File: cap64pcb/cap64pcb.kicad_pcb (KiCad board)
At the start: 2 copper layers, 91.6 x 12 mm, 29 parts, among them J1 SM05B_SURS_TF, Q1 BSS138, Q2 BSS138, U1 MPR121QR2, U2 SPX3819M5-L-3.3

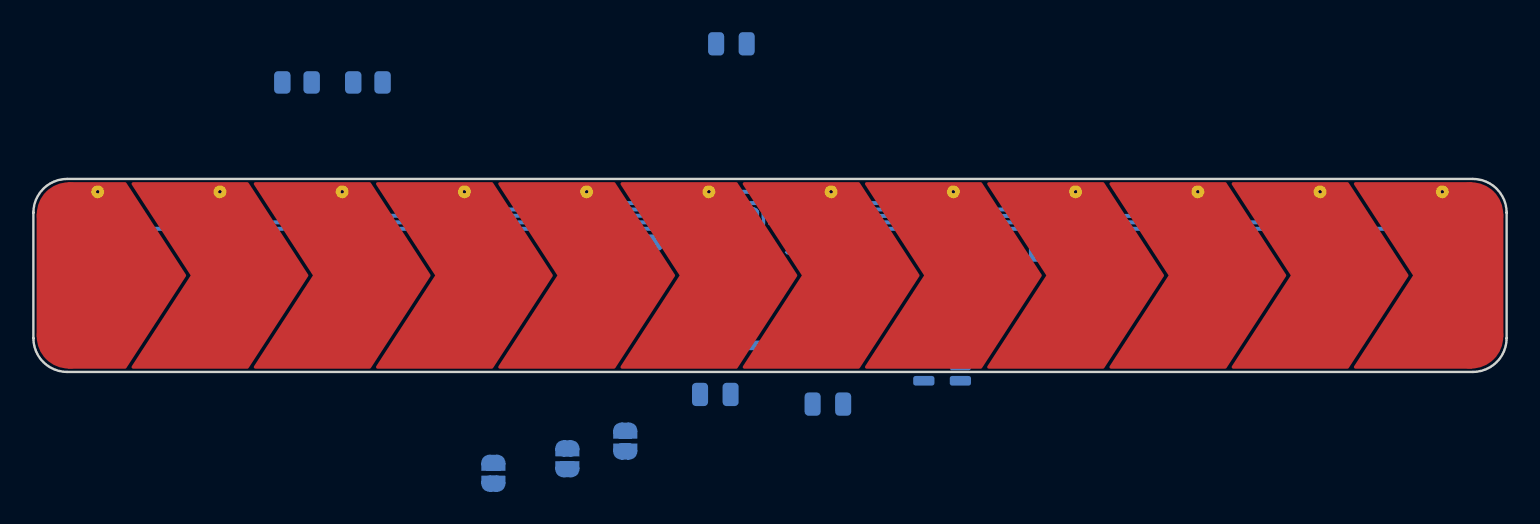
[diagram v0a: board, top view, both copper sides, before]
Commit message: test traces
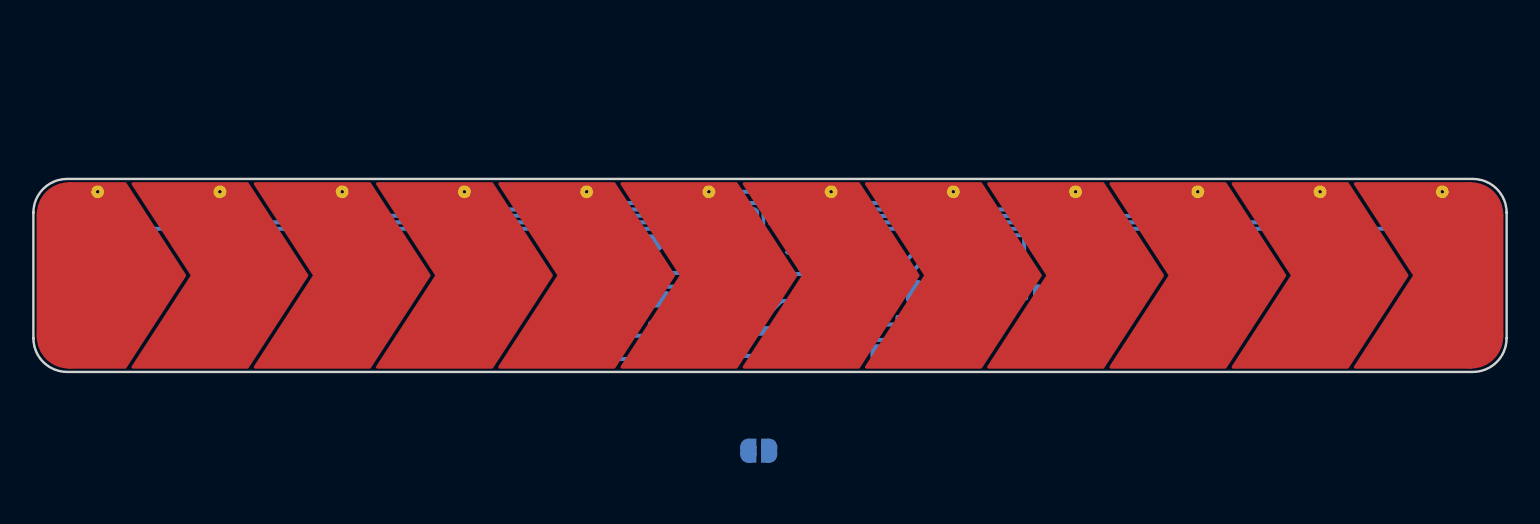
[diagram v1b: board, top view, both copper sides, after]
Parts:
- moved R2 34.7 mm to (83.2, 44.9), turned to -90 degrees
- moved R3 23.1 mm to (73.1, 47.4), turned to 90 degrees
- moved C3 18.0 mm to (77.3, 48.6), turned to -90 degrees
- moved JP1 10.6 mm to (68.1, 48.1), turned to 90 degrees
- moved JP2 9.68 mm to (70.7, 47.3), turned to 90 degrees
- moved JP3 8.32 mm to (79.3, 55.9), turned to 180 degrees
- moved C4 4.05 mm to (75.2, 48.6), turned to -90 degrees
- moved C2 3.72 mm to (85.8, 50.0)
- moved U2 2.20 mm to (89.6, 48.7)
- moved J1 2.15 mm to (95.8, 44.9)
- moved Q2 2.12 mm to (86.1, 45.5)
- moved C1 2.11 mm to (89.9, 46.0)
- moved Q1 1.03 mm to (80.3, 47.5)
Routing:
- net +3V3: track 0.00 -> 36.7 mm
- net GND: track 9.16 -> 45.8 mm
- net Net-(J1-Pad2): track 0.00 -> 19.0 mm
- net Net-(JP1-Pad2): track 0.00 -> 15.3 mm
- net Net-(J1-Pad3): track 0.00 -> 13.6 mm
- net SDA: track 0.00 -> 11.9 mm
- net Net-(C5-Pad1): track 0.00 -> 6.87 mm
- net SCL: track 0.00 -> 6.42 mm
- net VCC: track 0.00 -> 3.65 mm
- net Net-(C2-Pad1): track 0.00 -> 1.73 mm

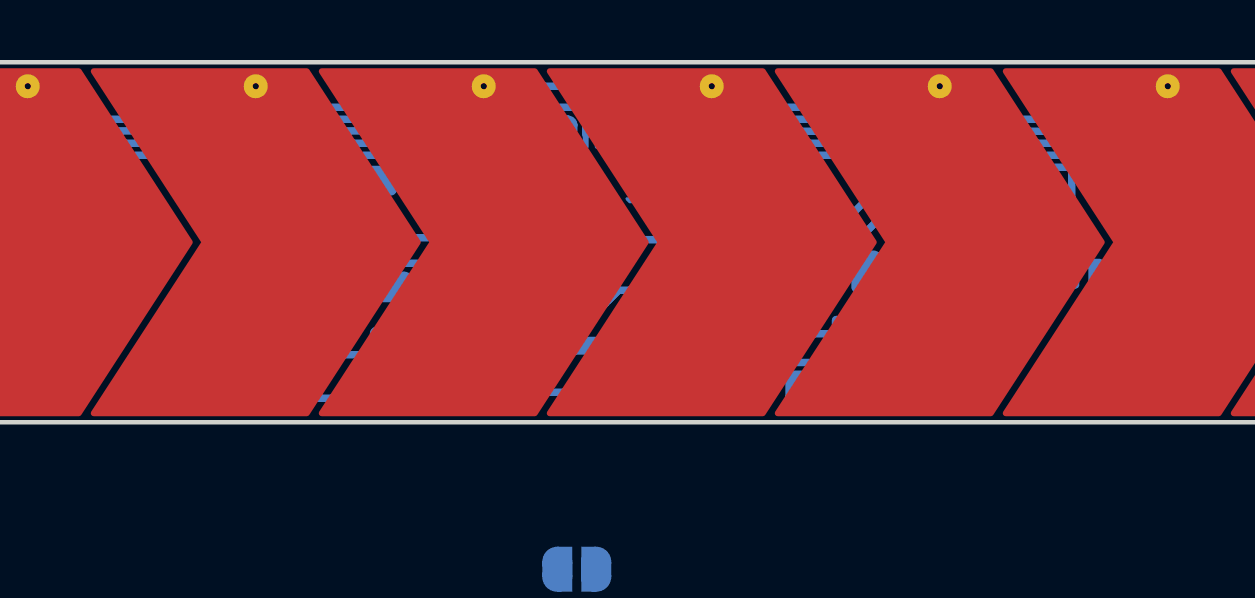
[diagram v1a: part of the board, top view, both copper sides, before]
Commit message: remove test traces
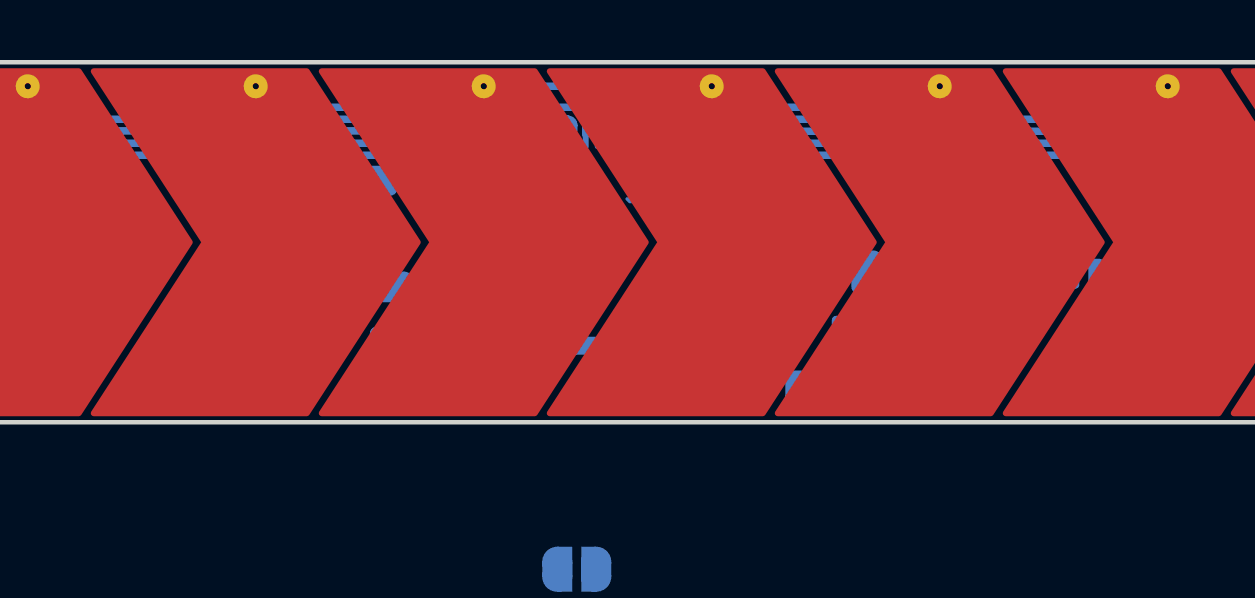
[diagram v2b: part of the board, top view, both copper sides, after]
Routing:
- net GND: track 45.8 -> 0.00 mm
- net +3V3: track 36.7 -> 0.00 mm
- net Net-(J1-Pad2): track 19.0 -> 0.00 mm
- net Net-(JP1-Pad2): track 15.3 -> 0.00 mm
- net Net-(J1-Pad3): track 13.6 -> 0.00 mm
- net SDA: track 11.9 -> 0.00 mm
- net Net-(C5-Pad1): track 6.87 -> 0.00 mm
- net SCL: track 6.42 -> 0.00 mm
- net VCC: track 3.65 -> 0.00 mm
- net Net-(R1-Pad1): track 2.14 -> 0.00 mm
- net Net-(C2-Pad1): track 1.73 -> 0.00 mm
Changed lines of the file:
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@@
   (gr_line (start 36.3 39) (end 123.7 39) (layer "Edge.Cuts") (width 0.15))
   (gr_line (start 125.8 48.9) (end 125.8 41.1) (layer "Edge.Cuts") (width 0.15))
-  (segment (start 90.7375 48.05) (end 91.85 48.05) (width 0.25) (layer "B.Cu") (net 1))
-  (segment (start 91.85 49.136219) (end 91.036219 49.95) (width 0.25) (layer "B.Cu") (net 1))
-  (segment (start 91.85 48.05) (end 91.85 49.136219) (width 0.25) (layer "B.Cu") (net 1))
-  (segment (start 91.036219 49.95) (end 90.7375 49.95) (width 0.25) (layer "B.Cu") (net 1))
-  (segment (start 89.38952 48.48952) (end 89.9 49) (width 0.25) (layer "B.Cu") (net 2))
-  (segment (start 77.3 49.55) (end 75.2 49.55) (width 0.25) (layer "B.Cu") (net 2))
-  (segment (start 77.75625 43.6) (end 77.15625 44.2) (width 0.25) (layer "B.Cu") (net 2))
-  (segment (start 85.83952 49.01048) (end 84.85 50) (width 0.25) (layer "B.Cu") (net 2))
-  (segment (start 70.3 43.15) (end 70.35 43.1) (width 0.25) (layer "B.Cu") (net 2))
-  (segment (start 89.38952 48.48952) (end 88.86856 49.01048) (width 0.25) (layer "B.Cu") (net 2))
-  (segment (start 77.75 50) (end 77.3 49.55) (width 0.25) (layer "B.Cu") (net 2))
-  (segment (start 70.35 43.1) (end 72.45 43.1) (width 0.25) (layer "B.Cu") (net 2))
-  (segment (start 66.2 46.925912) (end 69.975912 43.15) (width 0.25) (layer "B.Cu") (net 2))
-  (segment (start 77.15625 44.2) (end 75.7875 44.2) (width 0.25) (layer "B.Cu") (net 2))
-  (segment (start 75.2 49.55) (end 74.55 50.2) (width 0.25) (layer "B.Cu") (net 2))
-  (segment (start 69.975912 43.15) (end 70.3 43.15) (width 0.25) (layer "B.Cu") (net 2))
-  (segment (start 74.55 50.2) (end 67.3 50.2) (width 0.25) (layer "B.Cu") (net 2))
-  (segment (start 74.6875 43.1) (end 72.75 43.1) (width 0.25) (layer "B.Cu") (net 2))
-  (segment (start 89.9 49) (end 90.7375 49) (width 0.25) (layer "B.Cu") (net 2))
-  (segment (start 72.45 43.1) (end 72.6 42.95) (width 0.25) (layer "B.Cu") (net 2))
-  (segment (start 89.38952 46.63952) (end 89.38952 48.48952) (width 0.25) (layer "B.Cu") (net 2))
-  (segment (start 66.2 49.1) (end 66.2 46.925912) (width 0.25) (layer "B.Cu") (net 2))
-  (segment (start 88.86856 49.01048) (end 85.83952 49.01048) (width 0.25) (layer "B.Cu") (net 2))
-  (segment (start 67.3 50.2) (end 66.2 49.1) (width 0.25) (layer "B.Cu") (net 2))
-  (segment (start 72.75 43.1) (end 72.6 42.95) (width 0.25) (layer "B.Cu") (net 2))
-  (segment (start 78.6125 43.6) (end 77.75625 43.6) (width 0.25) (layer "B.Cu") (net 2))
-  (segment (start 84.85 50) (end 77.75 50) (width 0.25) (layer "B.Cu") (net 2))
-  (segment (start 88.95 46.2) (end 89.38952 46.63952) (width 0.25) (layer "B.Cu") (net 2))
-  (segment (start 75.7875 44.2) (end 74.6875 43.1) (width 0.25) (layer "B.Cu") (net 2))
-  (segment (start 88.4625 49.95) (end 86.8 49.95) (width 0.25) (layer "B.Cu") (net 3))
-  (segment (start 86.8 49.95) (end 86.75 50) (width 0.25) (layer "B.Cu") (net 3))
-  (segment (start 73.7625 47.65) (end 73.1 48.3125) (width 0.25) (layer "B.Cu") (net 4))
-  (segment (start 85.1625 46.45) (end 84.35 46.45) (width 0.25) (layer "B.Cu") (net 4))
-  (segment (start 79.3625 48.45) (end 78.1 48.45) (width 0.25) (layer "B.Cu") (net 4))
-  (segment (start 83.1 43.6) (end 81.3875 43.6) (width 0.25) (layer "B.Cu") (net 4))
-  (segment (start 78.1 48.45) (end 77.3 47.65) (width 0.25) (layer "B.Cu") (net 4))
-  (segment (start 83.2 48.5) (end 79.4125 48.5) (width 0.25) (layer "B.Cu") (net 4))
-  (segment (start 84.35 46.45) (end 83.8 47) (width 0.25) (layer "B.Cu") (net 4))
-  (segment (start 83.8 47) (end 82.3 47) (width 0.25) (layer "B.Cu") (net 4))
-  (segment (start 79.3625 47.9375) (end 79.3625 48.45) (width 0.25) (layer "B.Cu") (net 4))
-  (segment (start 79.4125 48.5) (end 79.3625 48.45) (width 0.25) (layer "B.Cu") (net 4))
-  (segment (start 72.6625 48.75) (end 68.1 48.75) (width 0.25) (layer "B.Cu") (net 4))
-  (segment (start 86.16452 44.871699) (end 86.16452 44.228301) (width 0.25) (layer "B.Cu") (net 4))
-  (segment (start 83.2 43.9875) (end 83.2 43.7) (width 0.25) (layer "B.Cu") (net 4))
-  (segment (start 86.16452 44.228301) (end 85.536219 43.6) (width 0.25) (layer "B.Cu") (net 4))
-  (segment (start 83.2 43.7) (end 83.1 43.6) (width 0.25) (layer "B.Cu") (net 4))
-  (segment (start 77.3 47.65) (end 75.2 47.65) (width 0.25) (layer "B.Cu") (net 4))
-  (segment (start 85.536219 43.6) (end 83.1 43.6) (width 0.25) (layer "B.Cu") (net 4))
-  (segment (start 81.9 46.6) (end 80.7 46.6) (width 0.25) (layer "B.Cu") (net 4))
-  (segment (start 83.65 48.05) (end 83.2 48.5) (width 0.25) (layer "B.Cu") (net 4))
-  (segment (start 82.3 47) (end 81.9 46.6) (width 0.25) (layer "B.Cu") (net 4))
-  (segment (start 75.2 47.65) (end 73.7625 47.65) (width 0.25) (layer "B.Cu") (net 4))
-  (segment (start 88.4625 48.05) (end 83.65 48.05) (width 0.25) (layer "B.Cu") (net 4))
-  (segment (start 80.7 46.6) (end 79.3625 47.9375) (width 0.25) (layer "B.Cu") (net 4))
-  (segment (start 73.1 48.3125) (end 72.6625 48.75) (width 0.25) (layer "B.Cu") (net 4))
-  (segment (start 85.1625 45.873719) (end 86.16452 44.871699) (width 0.25) (layer "B.Cu") (net 4))
-  (segment (start 85.1625 46.45) (end 85.1625 45.873719) (width 0.25) (layer "B.Cu") (net 4))
-  (segment (start 78.5375 44.85) (end 72.6 44.85) (width 0.25) (layer "B.Cu") (net 5))
-  (segment (start 79.2 44.1875) (end 78.5375 44.85) (width 0.25) (layer "B.Cu") (net 5))
-  (segment (start 87.53548 46.06452) (end 86.1 47.5) (width 0.25) (layer "B.Cu") (net 6))
-  (segment (start 88.03952 45.821699) (end 87.796699 46.06452) (width 0.25) (layer "B.Cu") (net 6))
-  (segment (start 95 42.9) (end 90.7 42.9) (width 0.25) (layer "B.Cu") (net 6))
-  (segment (start 90.7 42.9) (end 88.03952 45.56048) (width 0.25) (layer "B.Cu") (net 6))
-  (segment (start 87.796699 46.06452) (end 87.53548 46.06452) (width 0.25) (layer "B.Cu") (net 6))
-  (segment (start 95 42.9) (end 95 46.05) (width 0.25) (layer "B.Cu") (net 6))
-  (segment (start 86.1 47.5) (end 81.2375 47.5) (width 0.25) (layer "B.Cu") (net 6))
-  (segment (start 88.03952 45.56048) (end 88.03952 45.821699) (width 0.25) (layer "B.Cu") (net 6))
-  (segment (start 95.8 42.5) (end 95.8 46.05) (width 0.25) (layer "B.Cu") (net 7))
-  (segment (start 90.0375 42.5) (end 87.0375 45.5) (width 0.25) (layer "B.Cu") (net 7))
-  (segment (start 95.8 42.5) (end 90.0375 42.5) (width 0.25) (layer "B.Cu") (net 7))
-  (segment (start 70.8 45.7) (end 70.7 45.6) (width 0.25) (layer "B.Cu") (net 9))
-  (segment (start 70.7 46.65) (end 70.7 45.6) (width 0.25) (layer "B.Cu") (net 9))
-  (segment (start 70.7 44.85) (end 70.3 44.45) (width 0.25) (layer "B.Cu") (net 9))
-  (segment (start 70.7 46.65) (end 68.9 46.65) (width 0.25) (layer "B.Cu") (net 9))
-  (segment (start 68.9 46.65) (end 68.1 47.45) (width 0.25) (layer "B.Cu") (net 9))
-  (segment (start 78.8 45.7) (end 70.8 45.7) (width 0.25) (layer "B.Cu") (net 9))
-  (segment (start 79.6 44.9) (end 78.8 45.7) (width 0.25) (layer "B.Cu") (net 9))
-  (segment (start 70.7 45.6) (end 70.7 44.85) (width 0.25) (layer "B.Cu") (net 9))
-  (segment (start 79.6 44.1875) (end 79.6 44.9) (width 0.25) (layer "B.Cu") (net 9))
-  (segment (start 79.3625 46.55) (end 73.1625 46.55) (width 0.25) (layer "B.Cu") (net 10))
-  (segment (start 80 45.9125) (end 79.3625 46.55) (width 0.25) (layer "B.Cu") (net 10))
-  (segment (start 73.1 46.4875) (end 71.6375 47.95) (width 0.25) (layer "B.Cu") (net 10))
-  (segment (start 73.1625 46.55) (end 73.1 46.4875) (width 0.25) (layer "B.Cu") (net 10))
-  (segment (start 71.6375 47.95) (end 70.7 47.95) (width 0.25) (layer "B.Cu") (net 10))
-  (segment (start 80 44.1875) (end 80 45.9125) (width 0.25) (layer "B.Cu") (net 10))
-  (segment (start 83.18548 44.91452) (end 84.79798 44.91452) (width 0.25) (layer "B.Cu") (net 11))
-  (segment (start 83.2 44.92904) (end 83.18548 44.91452) (width 0.25) (layer "B.Cu") (net 11))
-  (segment (start 84.79798 44.91452) (end 85.1625 44.55) (width 0.25) (layer "B.Cu") (net 11))
-  (segment (start 83.2 45.8125) (end 83.2 44.92904) (width 0.25) (layer "B.Cu") (net 11))
-  (segment (start 80.4 44.1875) (end 80.4 44.700656) (width 0.25) (layer "B.Cu") (net 11))
-  (segment (start 80.4 44.700656) (end 80.613864 44.91452) (width 0.25) (layer "B.Cu") (net 11))
-  (segment (start 80.613864 44.91452) (end 83.18548 44.91452) (width 0.25) (layer "B.Cu") (net 11))
-  (segment (start 78.6125 43.2) (end 76.6125 43.2) (width 0.25) (layer "B.Cu") (net 12))
-  (segment (start 76.6125 43.2) (end 76.5125 43.1) (width 0.25) (layer "B.Cu") (net 12))
   (segment (start 38.2 40.3) (end 38.2 39.8) (width 0.25) (layer "B.Cu") (net 13))
   (segment (start 76.834315 42.1) (end 40 42.1) (width 0.25) (layer "B.Cu") (net 13))

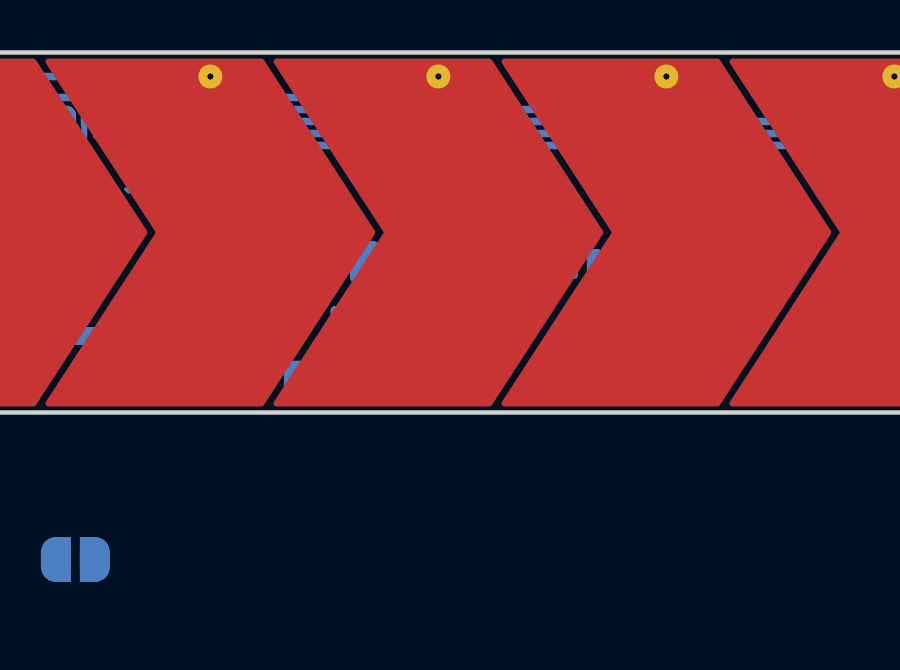
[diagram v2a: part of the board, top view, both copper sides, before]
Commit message: update pcb
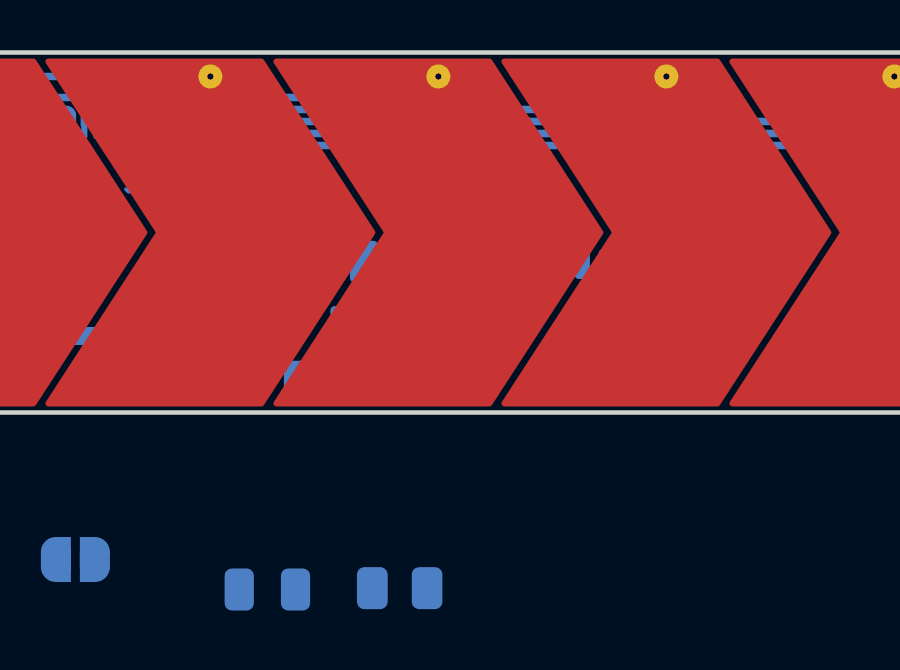
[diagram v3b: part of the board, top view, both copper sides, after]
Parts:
- added D1: RED, LED_SMD:LED_0805_2012Metric, B.Cu at (85.7, 56.9)
- added R4: 10kΩ, Resistor_SMD:R_0805_2012Metric, B.Cu at (90.1, 56.9)
- J1: footprint Connector_JST:JST_SUR_SM05B-SURS-TF_1x05-1MP_P0.80mm_Horizontal -> Connector_JST:JST_SUR_SM04B-SURS-TF_1x04-1MP_P0.80mm_Horizontal
- U2: value SPX3819M5-L-3.3 -> SPX3819M5-L-3-3
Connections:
- J1 pad 4: INT -> GND
- U1 pad 1: INT -> Net-(U1-Pad1)
